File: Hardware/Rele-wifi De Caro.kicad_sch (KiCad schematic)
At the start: 42 parts, among them J1 Screw_Terminal_01x03, J2 Screw_Terminal_01x03, J3 Screw_Terminal_01x03, J4 Screw_Terminal_01x03, J5 Screw_Terminal_01x02, K1 Relay_SPDT, K2 Relay_SPDT, K3 Relay_SPDT, K5 Relay_SPDT, Q1 BC547, Q2 PC817-B, Q3 BC547, Q4 PC817-B, Q5 PC817-B, Q6 BC547, Q7 PC817-B, Q8 BC547, U1 L7805, U2 ESP32-CAM, U3 LM7805_TO220

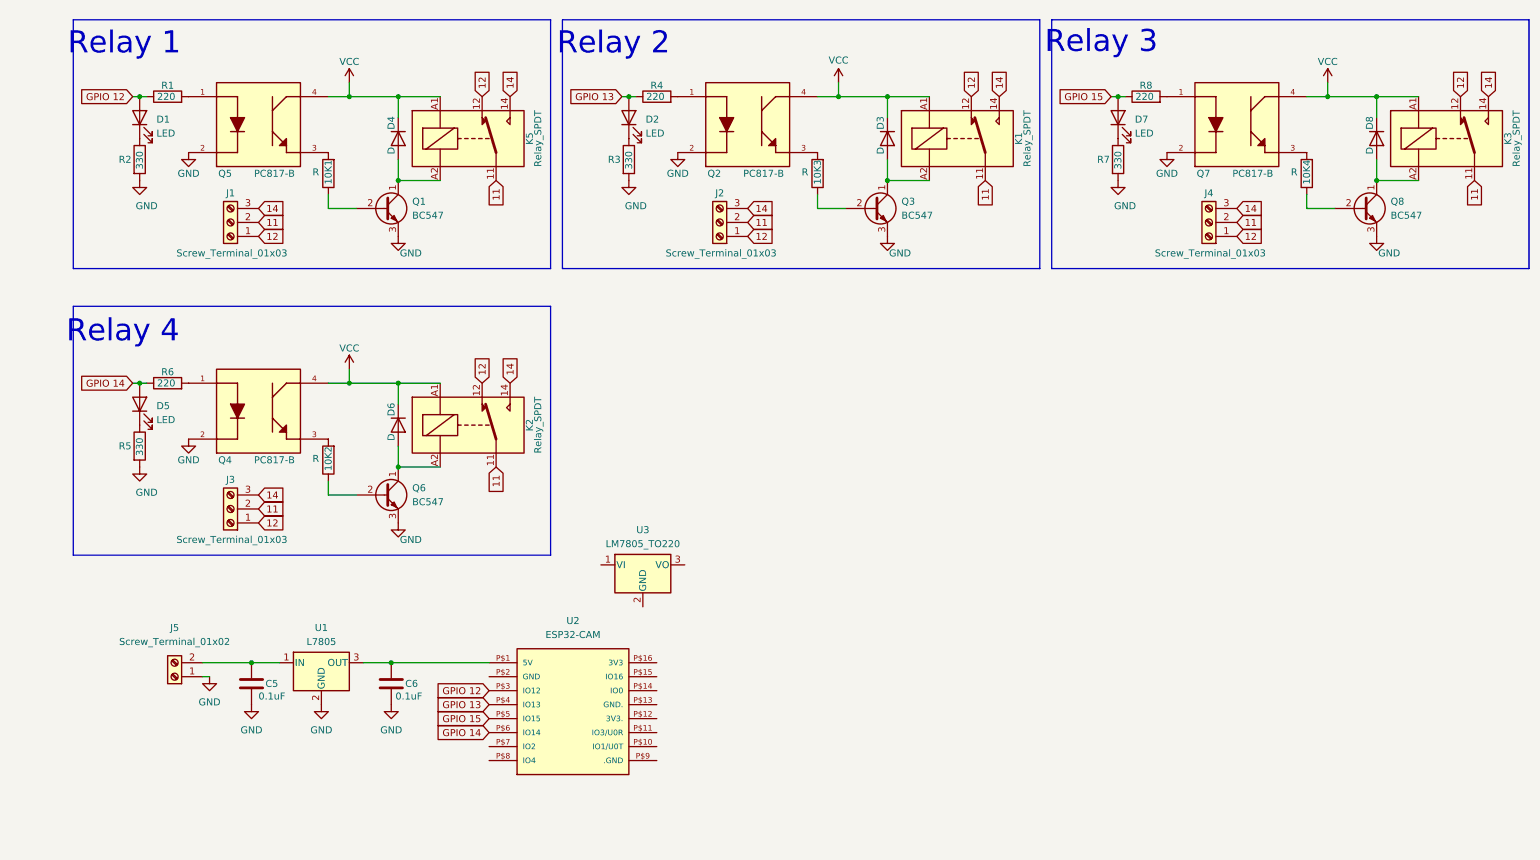
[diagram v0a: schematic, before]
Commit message: Avance de esquematico
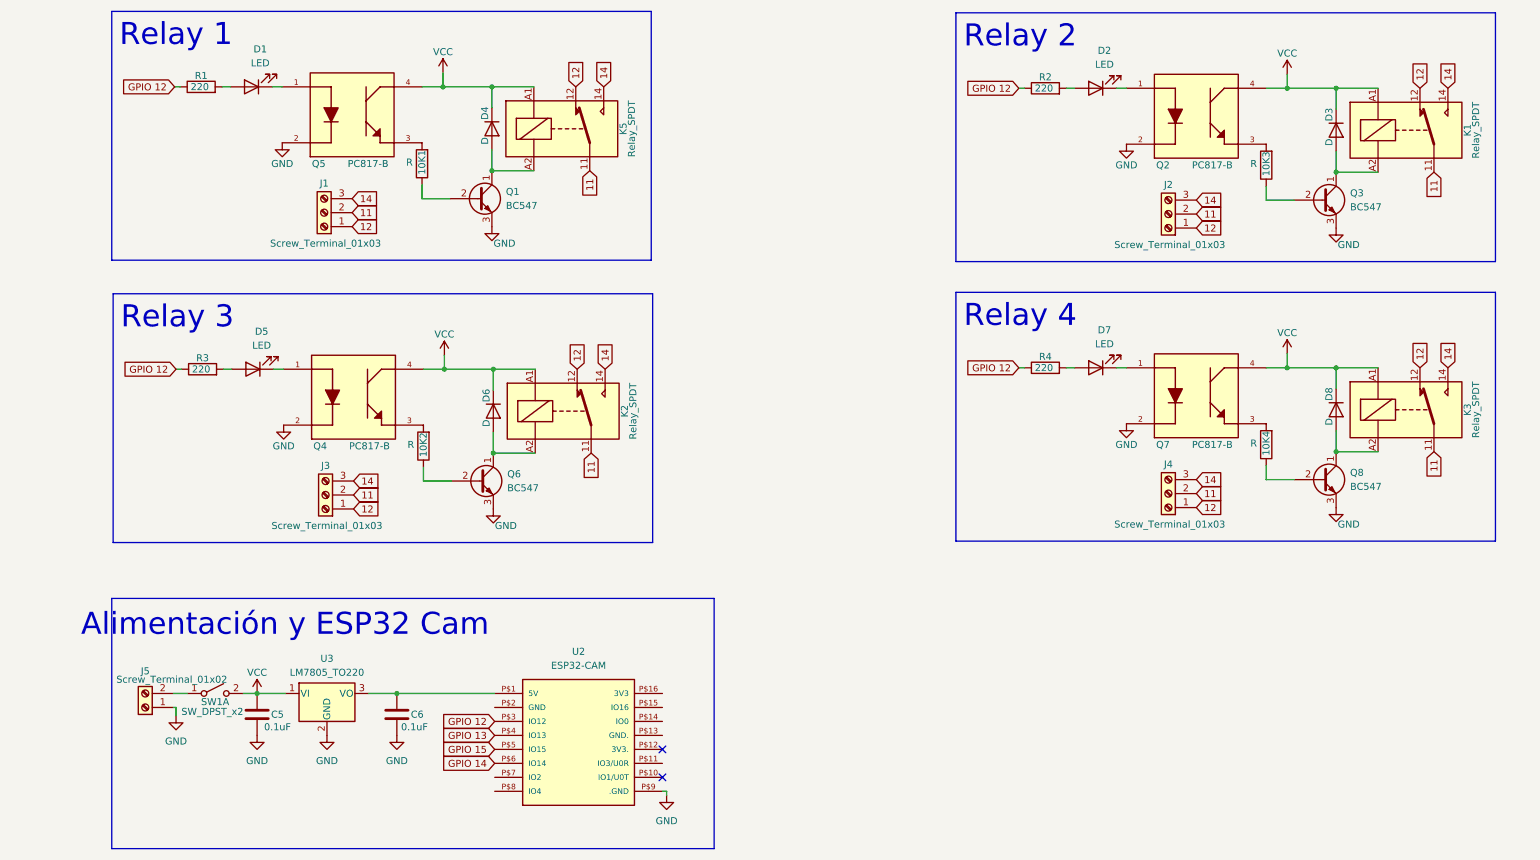
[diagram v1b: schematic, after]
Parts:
- removed R5, R7: 330, symbol Device:R
- removed R6, R8: 220, symbol Device:R
- removed U1: L7805, symbol Regulator_Linear:L7805
- added SW1: SW_DPST_x2, symbol Switch:SW_DPST_x2
- K1, K2, K3, K5: footprint (none) -> Relay:RELAY_PR13-5V-450-1C
- R2, R3: value 330 -> 220
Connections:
- net GND: now also U2.P$9 (.GND), U3.2 (GND); no longer R2.2, R3.2
- net GPIO 12: now also R2.1, R3.1, R4.1; no longer D1.2 (A)
- net GPIO 13: no longer D2.2 (A), R4.1
- net GPIO 14: no longer D5.2 (A)
- net GPIO 15: no longer D7.2 (A)
- net VCC: now also C5.1, U3.1 (VI), SW1.2 (B)
- net at R1.2: now also D1.2 (A); no longer Q5.1
- net at J5.2 (Pin_2): now also SW1.1 (A); no longer C5.1
- net at D2.1 (K): now also Q2.1; no longer R3.1
- net at R4.2: now also D7.2 (A); no longer Q2.1
- net at C6.1, U2.P$1 (5V): now also U3.3 (VO)
- net at D1.1 (K): now also Q5.1; no longer R2.1
- net at Q4.1: now also D5.1 (K)
- net at D7.1 (K): now also Q7.1
- new net: D2.2 (A), R2.2
- new net: D5.2 (A), R3.2
- no-connect marks 0 -> 2
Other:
- note added: "Alimentación y ESP32 Cam"
- moved on the sheet: 10K1, C5, C6, D1, D4, J1, J5, K5, Q1, Q5, R1, U2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

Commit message: Avance pcb
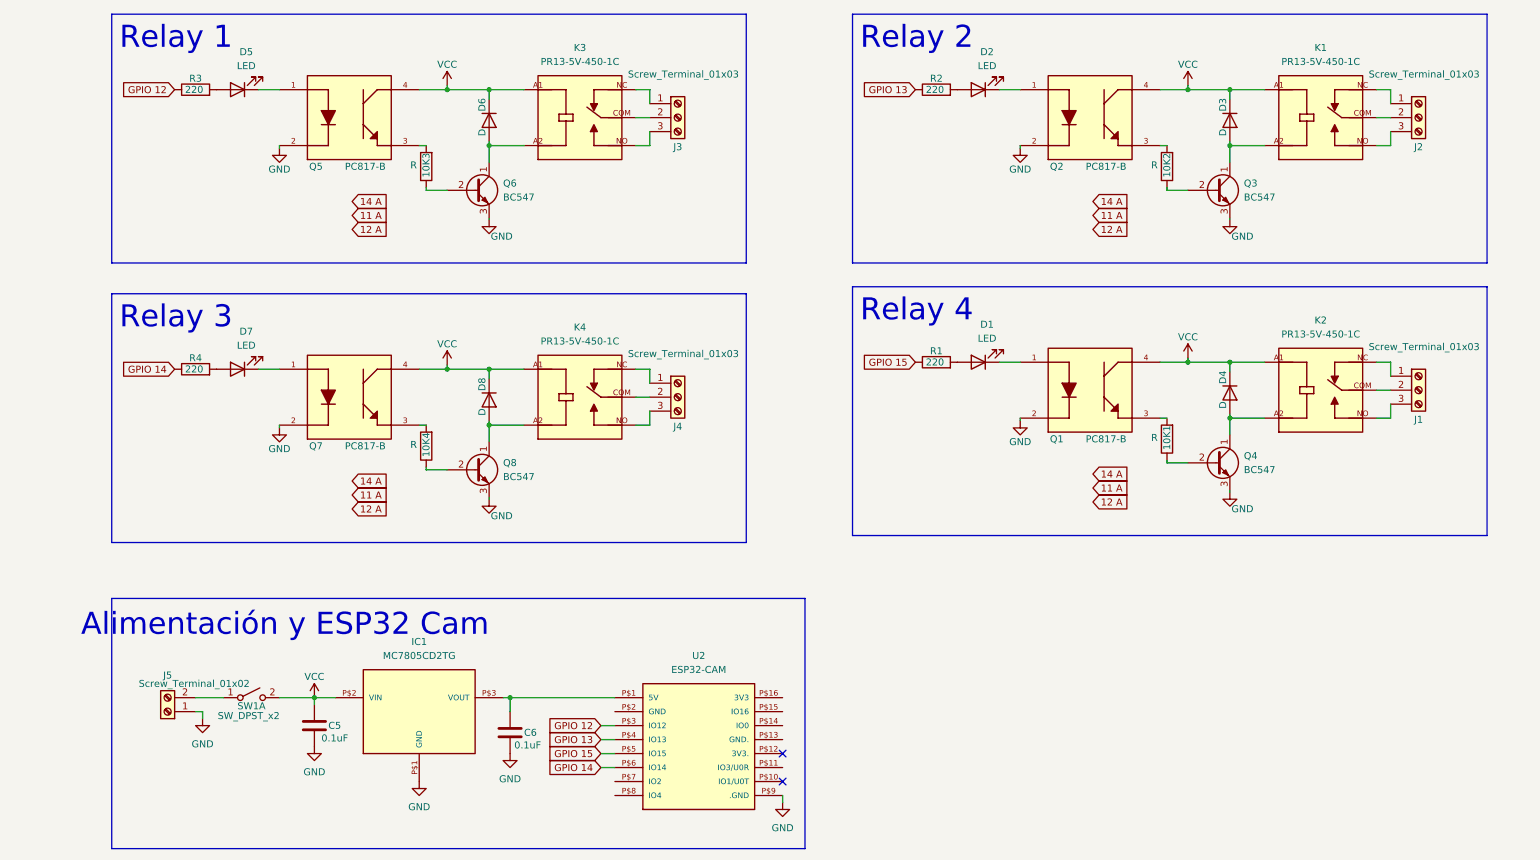
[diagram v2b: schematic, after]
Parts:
- removed K1, K2, K3, K5: Relay_SPDT, Relay:RELAY_PR13-5V-450-1C, symbol Relay:Relay_SPDT
- removed Q1: BC547, EESTN5:TO-92, symbol EESTN5:BC547
- removed Q4: PC817-B, Optocoplador:SOT254P1025X400-4N, symbol PC817-B:PC817-B
- removed U3: LM7805_TO220, Package_TO_SOT_THT:TO-220-3_Vertical, symbol Regulator_Linear:LM7805_TO220
- added IC1: MC7805CD2TG, 7805 d2pak:MC7805CD2TG, symbol 7805 d2pak:MC7805CD2TG
- added K1, K2, K3, K4: PR13-5V-450-1C, relay:RELAY_PR13-5V-450-1C, symbol relay:PR13-5V-450-1C
- added Q1: PC817-B, optoacoplador:SOT254P1025X400-4N, symbol PC817-B:PC817-B
- added Q4: BC547, bc547 smd:SOT95P230X110-3N, symbol EESTN5:BC547
- 10K1, 10K2, 10K3, 10K4, R1, R2, R3, R4: footprint (none) -> Resistor_SMD:R_0805_2012Metric_Pad1.20x1.40mm_HandSolder
- C5, C6: footprint (none) -> Capacitor_SMD:C_0805_2012Metric
- D1, D2, D5, D7: footprint (none) -> LED_SMD:LED_0805_2012Metric
- D3, D4, D6, D8: footprint (none) -> Diode_SMD:D_0805_2012Metric
- Q2, Q5, Q7: footprint Optocoplador:SOT254P1025X400-4N -> optoacoplador:SOT254P1025X400-4N
- Q3, Q6, Q8: footprint EESTN5:TO-92 -> bc547 smd:SOT95P230X110-3N
- U2: footprint ESP32 cam:ESP32-CAM -> esp cam:ESP32-CAM
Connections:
- net GND: now also IC1.P$1 (GND), Q1.2, Q4.3 (E)
- net GPIO 12: no longer R1.1, R2.1, R4.1
- net GPIO 13: now also R2.1
- net GPIO 14: now also R4.1
- net GPIO 15: now also R1.1
- net VCC: now also IC1.P$2 (VIN), K1.A1, K2.A1, K3.A1, K4.A1, Q1.4
- net at D4.2 (A): now also K2.A2, Q4.1 (C)
- net at 10K2.1: now also Q3.2 (B); no longer Q6.2 (B)
- net at 10K2.2: now also Q2.3
- net at 10K1.1: now also Q4.2 (B)
- net at D5.1 (K): now also Q5.1
- net at D8.2 (A), Q8.1 (C): now also K4.A2
- net at D1.1 (K): now also Q1.1; no longer Q5.1
- net at 10K1.2: now also Q1.3; no longer Q5.3
- net at 10K3.1: now also Q6.2 (B); no longer Q3.2 (B)
- net at 10K3.2: now also Q5.3; no longer Q2.3
- net at C6.1, U2.P$1 (5V): now also IC1.P$3 (VOUT)
- net at D6.2 (A), Q6.1 (C): now also K3.A2
- net at D3.2 (A), Q3.1 (C): now also K1.A2
- removed net 11: J1.2 (Pin_2), J2.2 (Pin_2), J3.2 (Pin_2), J4.2 (Pin_2)
- removed net 12: J1.1 (Pin_1), J2.1 (Pin_1), J3.1 (Pin_1), J4.1 (Pin_1)
- removed net 14: J1.3 (Pin_3), J2.3 (Pin_3), J3.3 (Pin_3), J4.3 (Pin_3)
- new net: J2.2 (Pin_2), K1.COM
- new net: J2.1 (Pin_1), K1.NC
- new net: J2.3 (Pin_3), K1.NO
- new net: J4.2 (Pin_2), K4.COM
- new net: J4.1 (Pin_1), K4.NC
- new net: J4.3 (Pin_3), K4.NO
- new net: J1.2 (Pin_2), K2.COM
- new net: J1.1 (Pin_1), K2.NC
- new net: J1.3 (Pin_3), K2.NO
- new net: J3.2 (Pin_2), K3.COM
- new net: J3.1 (Pin_1), K3.NC
- new net: J3.3 (Pin_3), K3.NO
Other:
- moved on the sheet: C5, C6, J5, SW1A, U2
